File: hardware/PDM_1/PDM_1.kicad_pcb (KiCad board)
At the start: 4 copper layers, 55 x 100 mm, 147 parts, among them IC2 BTS722204ESAXUMA1, IC3 BTS722204ESAXUMA1, IC4 BTS722204ESAXUMA1, IC5 BTS722204ESAXUMA1, J1 FTSH-107-01-L-DV-K-A, J2 UPT-08-01-01-L-RA, J5 UPT-02-01-01-X-RA, J6 Conn_01x06, J7 UPT-08-01-01-L-RA, U1 STM32G0C1KCTxN, U2 LD1117S33TR_SOT223, U3 LM2675M-5.0/NOPB, U5 MCP2542FDxMF

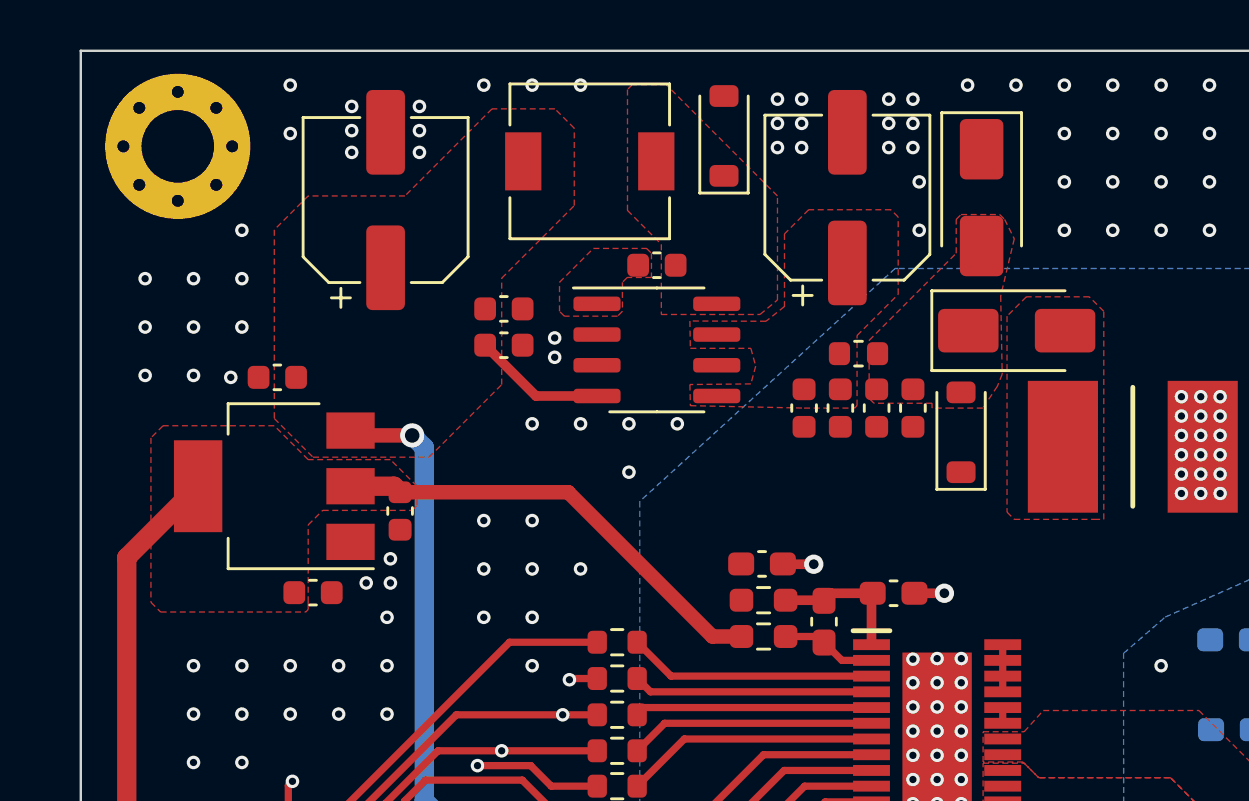
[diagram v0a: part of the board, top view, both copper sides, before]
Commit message: Poprawki 3
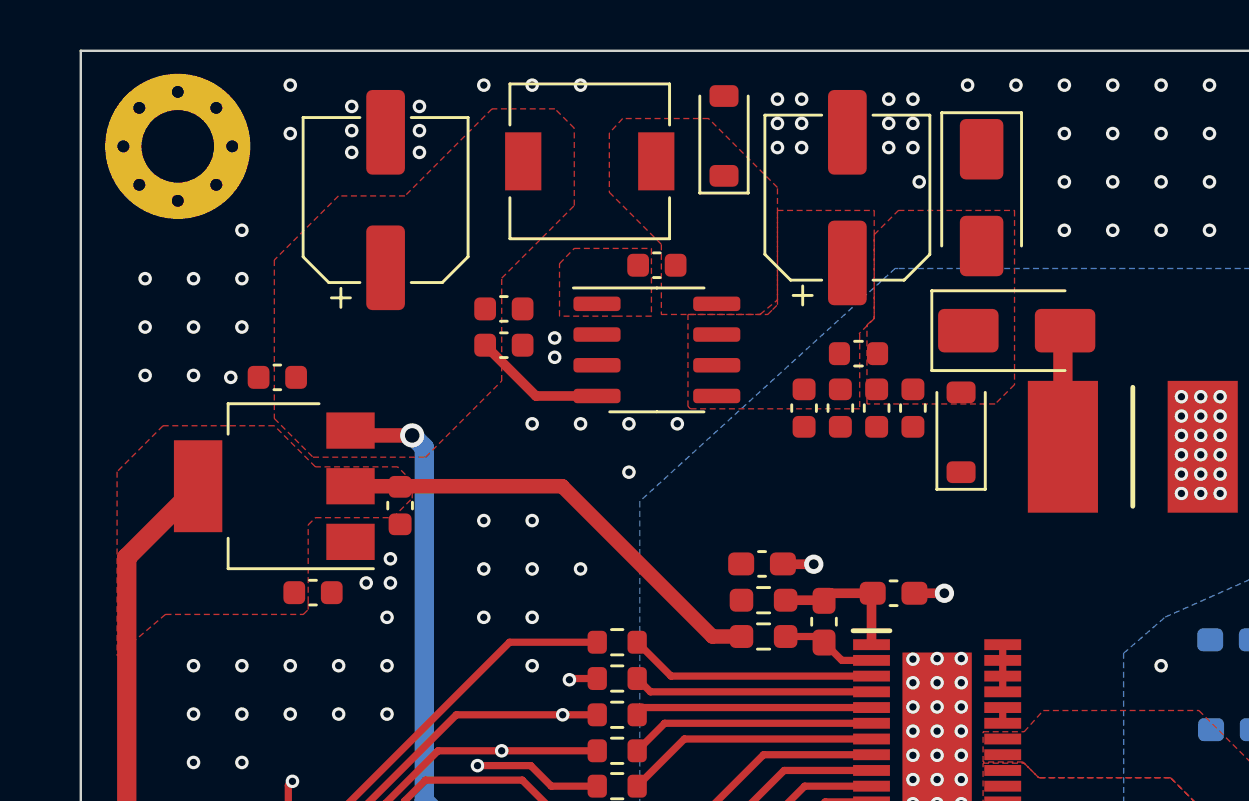
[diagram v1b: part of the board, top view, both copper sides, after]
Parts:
- moved C11 0.23 mm to (138.2, 78.8)
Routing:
- net /power/VIN: track 0.00 -> 4.84 mm
- net GND: vias 226 -> 225
- removed copper zone on F.Cu, net /power/VIN

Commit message: Poprawki 4
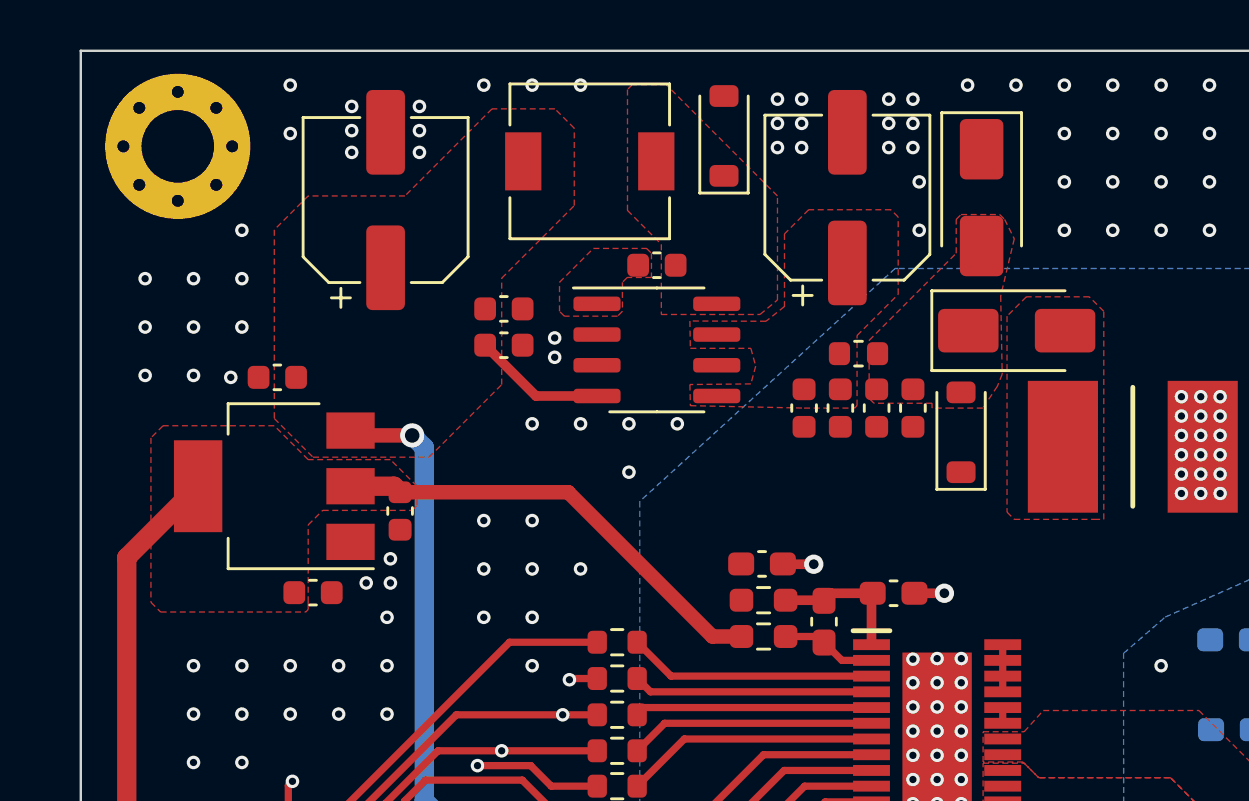
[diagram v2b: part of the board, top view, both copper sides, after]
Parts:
- moved C11 0.23 mm to (138.2, 79.0)
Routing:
- net /power/VIN: track 4.84 -> 0.00 mm
- net GND: vias 225 -> 226
- added copper zone on F.Cu, net /power/VIN

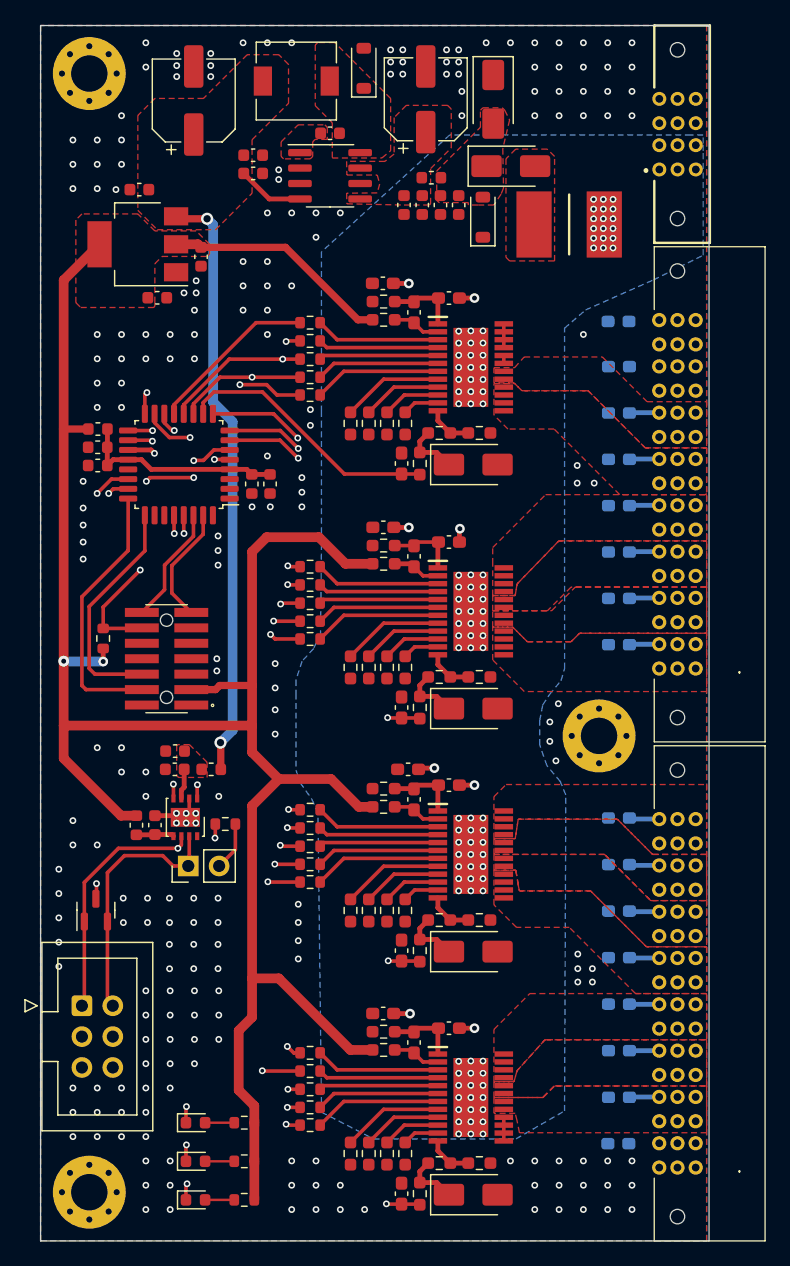
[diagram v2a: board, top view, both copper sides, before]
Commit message: Poprawki 5
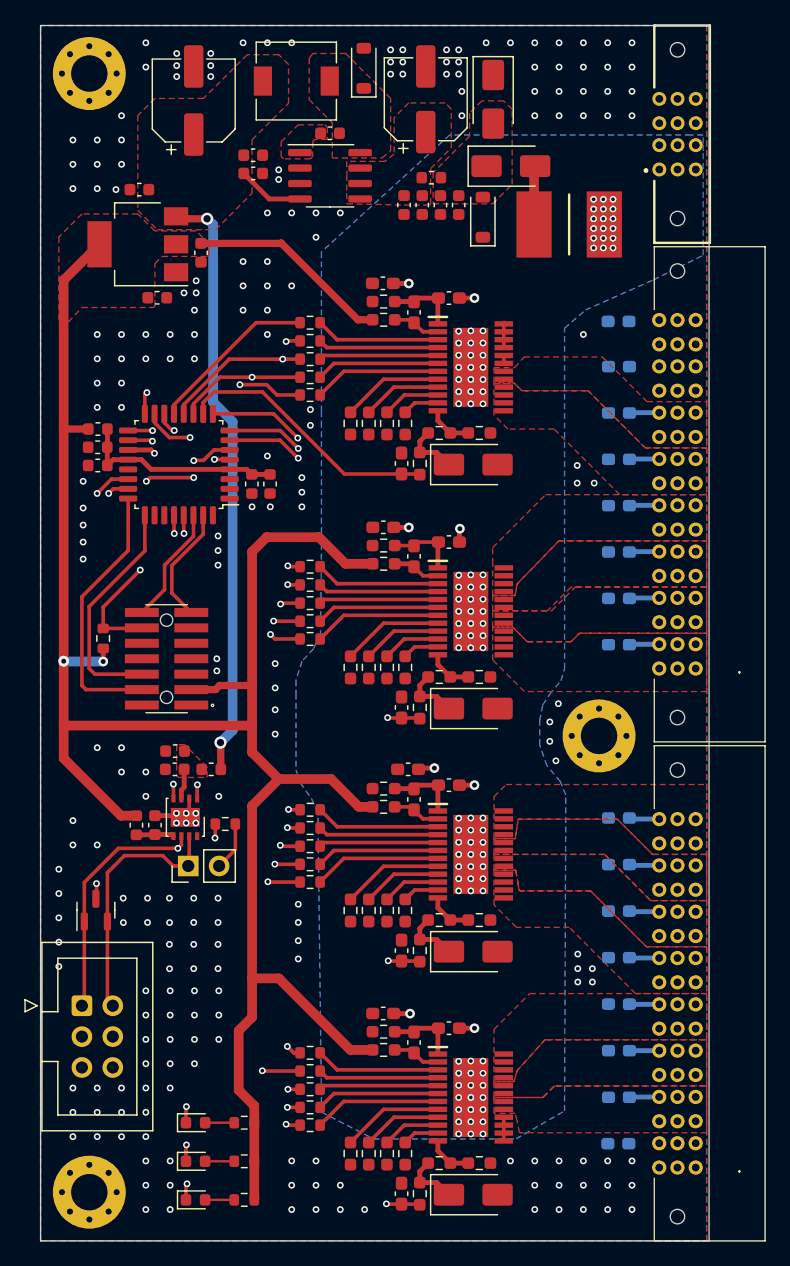
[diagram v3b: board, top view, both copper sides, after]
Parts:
- moved C11 0.33 mm to (138.2, 78.7)
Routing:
- net /power/VIN: track 0.00 -> 4.84 mm
- net +3.3V: track 185.7 -> 183.7 mm
- removed copper zone on F.Cu, net /power/VIN
